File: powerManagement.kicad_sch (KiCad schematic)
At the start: 24 parts, among them IC1 AP2112K-3.3, IC2 MPQ4420HGJ-Z

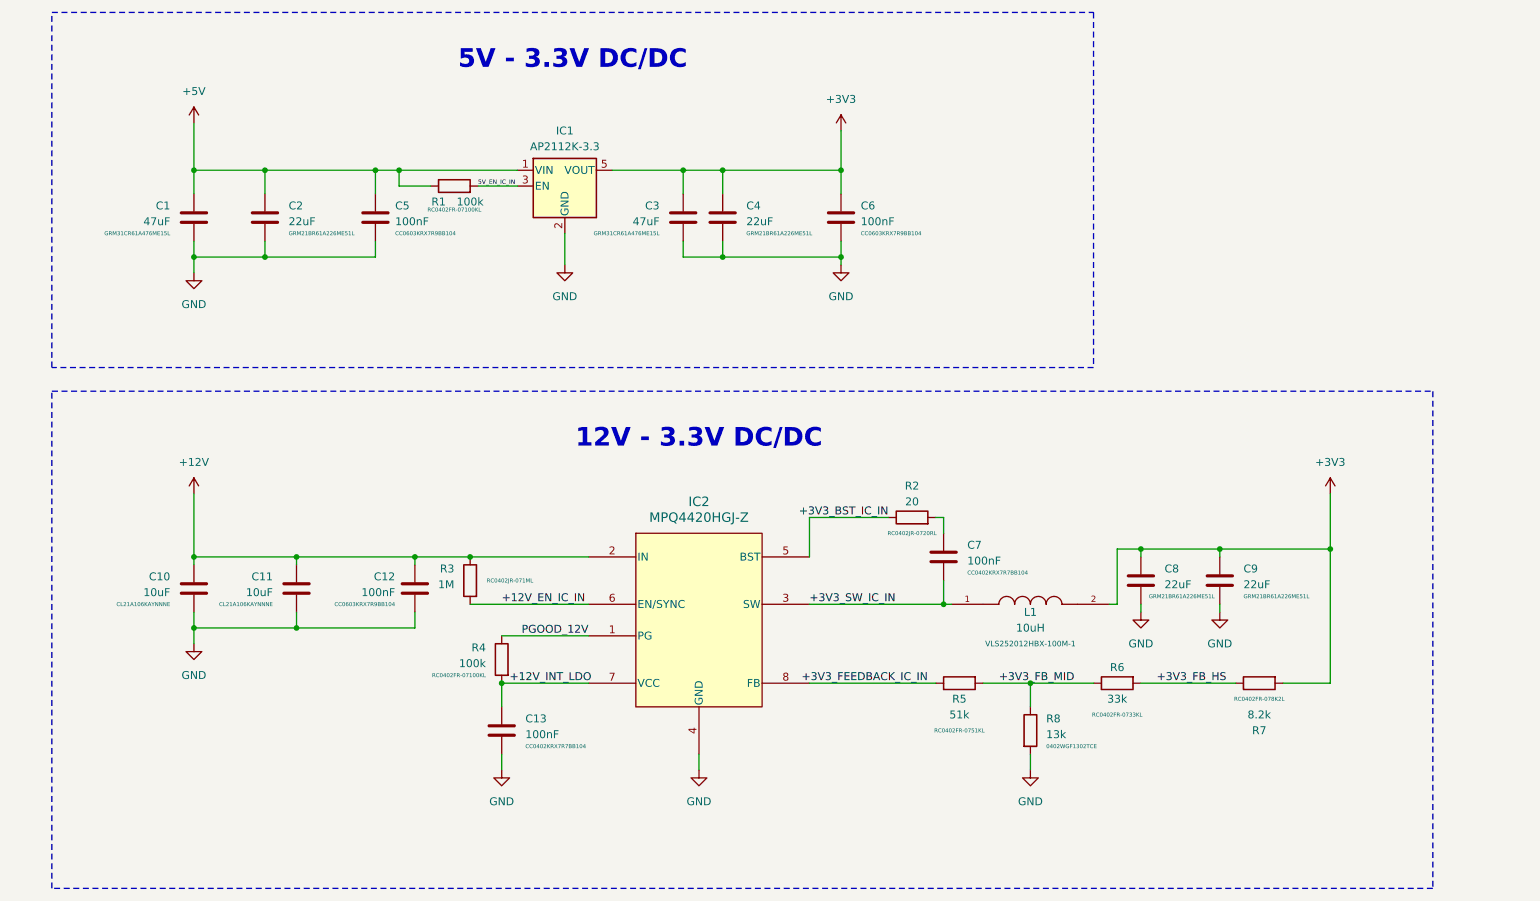
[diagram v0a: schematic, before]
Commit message: Changes to final schematic
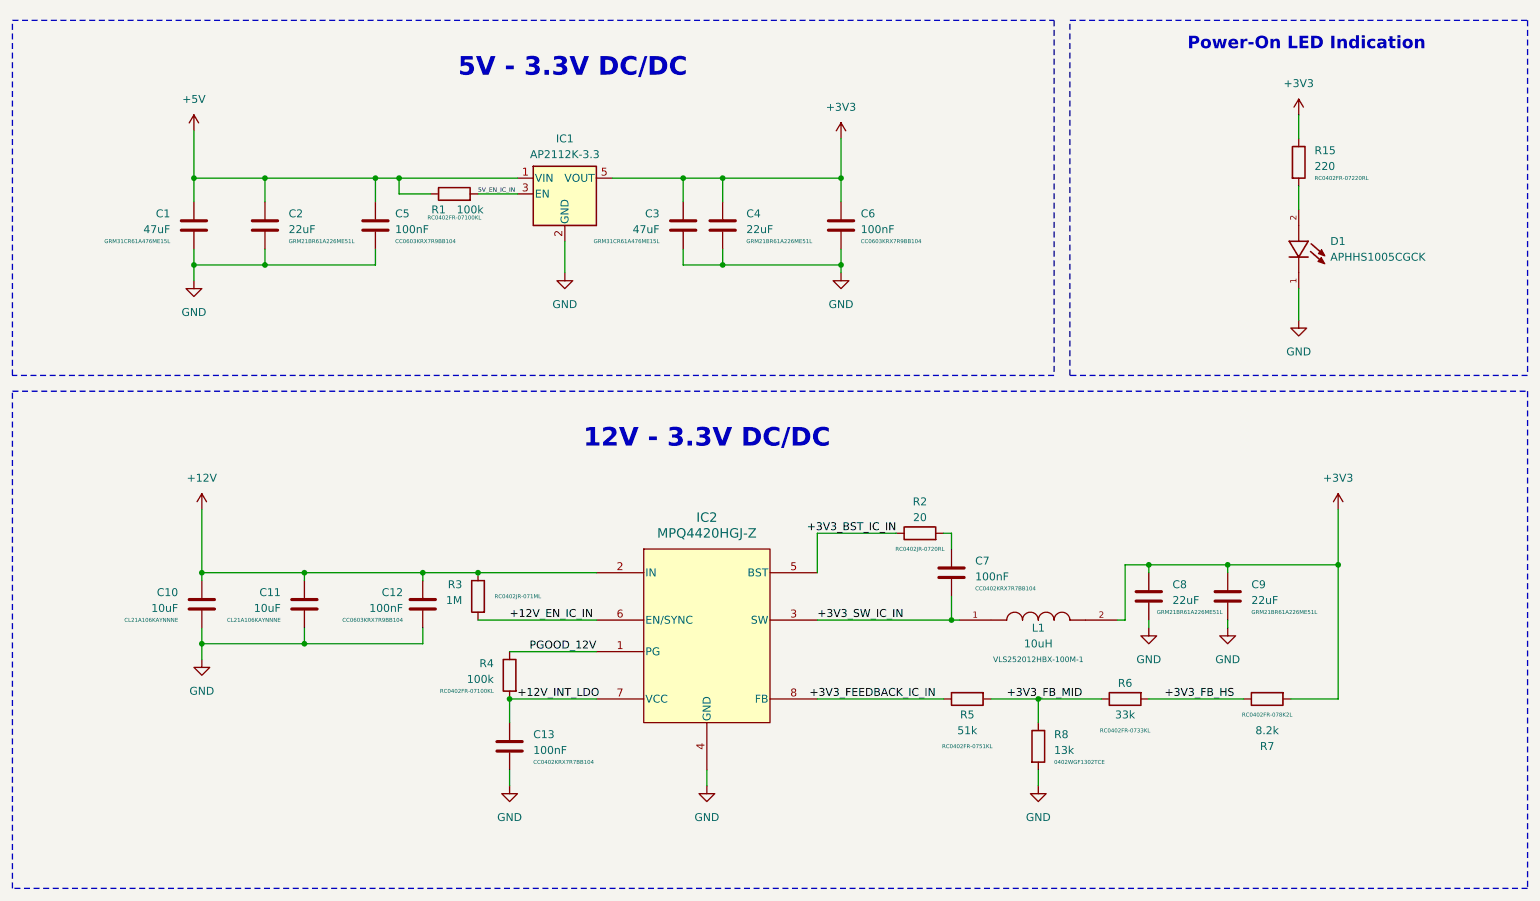
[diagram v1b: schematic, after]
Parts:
- added D1: APHHS1005CGCK, APHHS1005CGCK:LED_APHHS1005CGCK, symbol APHHS1005CGCK:APHHS1005CGCK
- added R15: 220, RC0402FR-07220RL:RESC1005X40N, symbol Project_Resistors:RC0402FR-07220RL
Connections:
- net +3V3: now also R15.1
- net GND: now also D1.1
- new net: D1.2, R15.2
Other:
- note added: "Power-On LED Indication"
- moved on the sheet: C1, C10, C11, C12, C13, C2, C3, C4, C5, C6, C7, C8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
